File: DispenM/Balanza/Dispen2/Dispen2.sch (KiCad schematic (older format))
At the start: 13 parts, among them M1 Motor_Servo, U1 LoRa32U4, U2 DS3231MZ

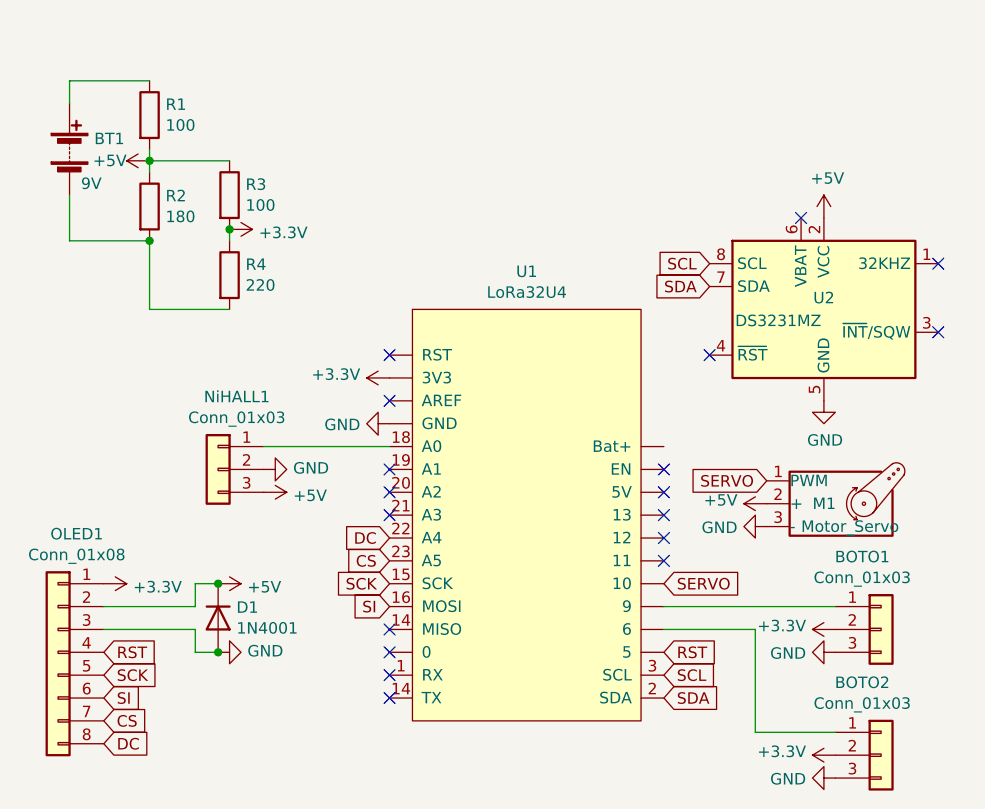
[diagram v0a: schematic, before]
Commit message: Actualizacion software y pcb
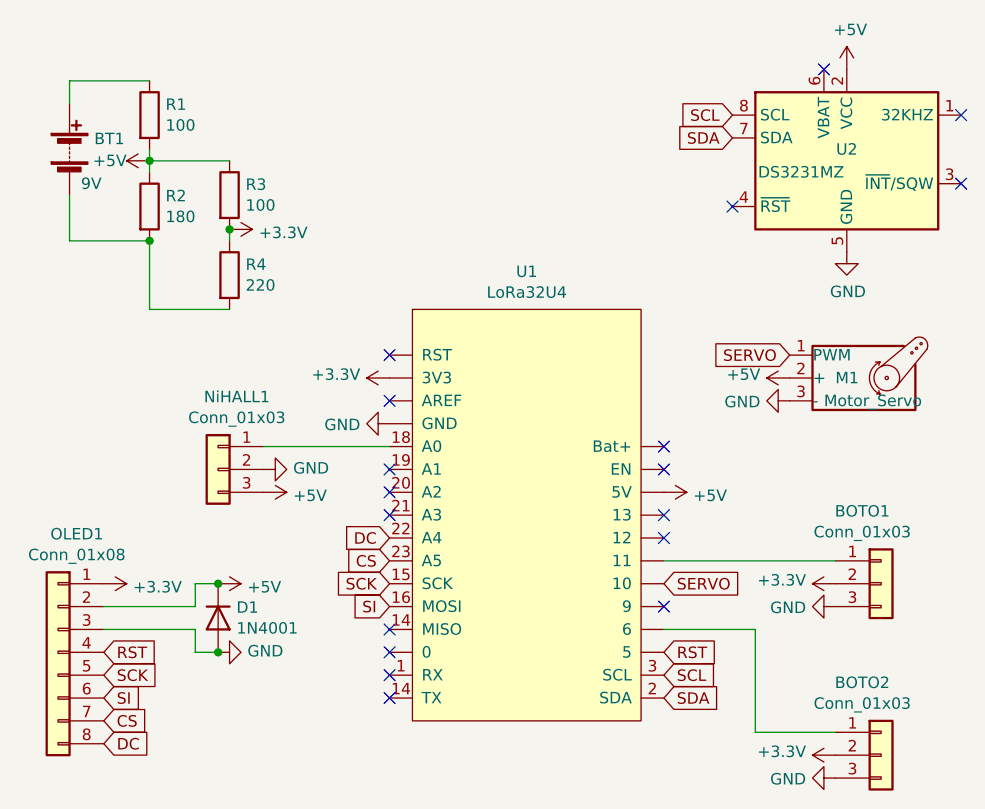
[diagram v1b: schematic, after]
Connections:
- net +5V: now also U1.~ (RST)
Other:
- moved on the sheet: BOTO1, M1, U2
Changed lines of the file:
@@
 $EndDescr
-$Comp
-L LoRa32U4:LoRa32U4 U1
-U 1 1 64849BFA
-P 5200 2750
-F 0 "U1" H 5200 3515 50  0000 C CNN
-F 1 "LoRa32U4" H 5200 3424 50  0000 C CNN
-F 2 "MODULOS:Lora32U4" H 5200 2750 50  0001 C CNN
-F 3 "" H 5200 2750 50  0001 C CNN
-	1    5200 2750
-	1    0    0    -1
-$EndComp
 $Comp
 L Motor:Motor_Servo M1
 U 1 1 6484B47B
-P 6550 3000
-F 0 "M1" H 6450 3000 50  0000 L CNN
-F 1 "Motor_Servo" H 6400 2900 50  0000 L CNN
-F 2 "Connector_PinHeader_2.54mm:PinHeader_1x03_P2.54mm_Vertical" H 6550 2810 50  0001 C CNN
-F 3 "http://forums.parallax.com/uploads/attachments/46831/74481.png" H 6550 2810 50  0001 C CNN
-	1    6550 3000
+P 6650 2450
+F 0 "M1" H 6550 2450 50  0000 L CNN
+F 1 "Motor_Servo" H 6500 2350 50  0000 L CNN
+F 2 "Connector_PinHeader_2.54mm:PinHeader_1x03_P2.54mm_Vertical" H 6650 2260 50  0001 C CNN
+F 3 "http://forums.parallax.com/uploads/attachments/46831/74481.png" H 6650 2260 50  0001 C CNN
+	1    6650 2450
 	1    0    0    -1
 $EndComp
@@
 L Timer_RTC:DS3231MZ U2
 U 1 1 6484C580
-P 6500 2150
-F 0 "U2" H 6500 2200 50  0000 C CNN
-F 1 "DS3231MZ" H 6300 2100 50  0000 C CNN
-F 2 "MODULOS:DS3231MH" H 6500 1650 50  0001 C CNN
-F 3 "http://datasheets.maximintegrated.com/en/ds/DS3231M.pdf" H 6500 1550 50  0001 C CNN
-	1    6500 2150
+P 6600 1500
+F 0 "U2" H 6600 1550 50  0000 C CNN
+F 1 "DS3231MZ" H 6400 1450 50  0000 C CNN
+F 2 "MODULOS:DS3231MH" H 6600 1000 50  0001 C CNN
+F 3 "http://datasheets.maximintegrated.com/en/ds/DS3231M.pdf" H 6600 900 50  0001 C CNN
+	1    6600 1500
 	1    0    0    -1
 $EndComp
@@
 L Connector_Generic:Conn_01x03 BOTO1
 U 1 1 6484ED92
-P 6750 3550
-F 0 "BOTO1" H 6668 3867 50  0000 C CNN
-F 1 "Conn_01x03" H 6668 3776 50  0000 C CNN
-F 2 "Connector_PinHeader_2.54mm:PinHeader_1x03_P2.54mm_Vertical" H 6750 3550 50  0001 C CNN
-F 3 "~" H 6750 3550 50  0001 C CNN
-	1    6750 3550
+P 6750 3350
+F 0 "BOTO1" H 6668 3667 50  0000 C CNN
+F 1 "Conn_01x03" H 6668 3576 50  0000 C CNN
+F 2 "Connector_PinHeader_2.54mm:PinHeader_1x03_P2.54mm_Vertical" H 6750 3350 50  0001 C CNN
+F 3 "~" H 6750 3350 50  0001 C CNN
+	1    6750 3350
 	1    0    0    -1
 $EndComp
@@
 L power:+3.3V #PWR0102
 U 1 1 648545ED
-P 6550 3550
-F 0 "#PWR0102" H 6550 3400 50  0001 C CNN
-F 1 "+3.3V" V 6565 3678 50  0000 L CNN
-F 2 "" H 6550 3550 50  0001 C CNN
-F 3 "" H 6550 3550 50  0001 C CNN
-	1    6550 3550
+P 6550 3350
+F 0 "#PWR0102" H 6550 3200 50  0001 C CNN
+F 1 "+3.3V" V 6565 3478 50  0000 L CNN
+F 2 "" H 6550 3350 50  0001 C CNN
+F 3 "" H 6550 3350 50  0001 C CNN
+	1    6550 3350
 	0    -1   -1   0
 $EndComp
@@
 L power:+5V #PWR0104
 U 1 1 64856200
-P 6250 3000
-F 0 "#PWR0104" H 6250 2850 50  0001 C CNN
-F 1 "+5V" V 6265 3128 50  0000 L CNN
-F 2 "" H 6250 3000 50  0001 C CNN
-F 3 "" H 6250 3000 50  0001 C CNN
-	1    6250 3000
+P 6350 2450
+F 0 "#PWR0104" H 6350 2300 50  0001 C CNN
+F 1 "+5V" V 6365 2578 50  0000 L CNN
+F 2 "" H 6350 2450 50  0001 C CNN
+F 3 "" H 6350 2450 50  0001 C CNN
+	1    6350 2450
 	0    -1   -1   0
 $EndComp
@@
 L power:+5V #PWR0105
 U 1 1 64856E0D
-P 6500 1750
-F 0 "#PWR0105" H 6500 1600 50  0001 C CNN
-F 1 "+5V" H 6515 1923 50  0000 C CNN
-F 2 "" H 6500 1750 50  0001 C CNN
-F 3 "" H 6500 1750 50  0001 C CNN
-	1    6500 1750
+P 6600 1100
+F 0 "#PWR0105" H 6600 950 50  0001 C CNN
+F 1 "+5V" H 6615 1273 50  0000 C CNN
+F 2 "" H 6600 1100 50  0001 C CNN
+F 3 "" H 6600 1100 50  0001 C CNN
+	1    6600 1100
 	1    0    0    -1
 $EndComp
@@
 	0    1    1    0
 $EndComp
-NoConn ~ 7000 1950
-NoConn ~ 7000 2250
-NoConn ~ 6000 2350
+NoConn ~ 7100 1300
+NoConn ~ 7100 1600
+NoConn ~ 6100 1700
 $Comp
 L power:GND #PWR0107
@@
 L power:GND #PWR0109
 U 1 1 6485B66E
-P 6500 2550
-F 0 "#PWR0109" H 6500 2300 50  0001 C CNN
-F 1 "GND" H 6505 2377 50  0000 C CNN
-F 2 "" H 6500 2550 50  0001 C CNN
-F 3 "" H 6500 2550 50  0001 C CNN
-	1    6500 2550
+P 6600 1900
+F 0 "#PWR0109" H 6600 1650 50  0001 C CNN
+F 1 "GND" H 6605 1727 50  0000 C CNN
+F 2 "" H 6600 1900 50  0001 C CNN
+F 3 "" H 6600 1900 50  0001 C CNN
+	1    6600 1900
 	1    0    0    -1
 $EndComp
@@
 L power:GND #PWR0110
 U 1 1 6485BFB9
-P 6550 3650
-F 0 "#PWR0110" H 6550 3400 50  0001 C CNN
-F 1 "GND" V 6555 3522 50  0000 R CNN
-F 2 "" H 6550 3650 50  0001 C CNN
-F 3 "" H 6550 3650 50  0001 C CNN
-	1    6550 3650
+P 6550 3450
+F 0 "#PWR0110" H 6550 3200 50  0001 C CNN
+F 1 "GND" V 6555 3322 50  0000 R CNN
+F 2 "" H 6550 3450 50  0001 C CNN
+F 3 "" H 6550 3450 50  0001 C CNN
+	1    6550 3450
 	0    1    1    0
 $EndComp
@@
 L power:GND #PWR0112
 U 1 1 6485CF38
-P 6250 3100
-F 0 "#PWR0112" H 6250 2850 50  0001 C CNN
-F 1 "GND" V 6255 2972 50  0000 R CNN
-F 2 "" H 6250 3100 50  0001 C CNN
-F 3 "" H 6250 3100 50  0001 C CNN
-	1    6250 3100
+P 6350 2550
+F 0 "#PWR0112" H 6350 2300 50  0001 C CNN
+F 1 "GND" V 6355 2422 50  0000 R CNN
+F 2 "" H 6350 2550 50  0001 C CNN
+F 3 "" H 6350 2550 50  0001 C CNN
+	1    6350 2550
 	0    1    1    0
 $EndComp
@@
 Text GLabel 5800 3350 2    50   Input ~ 0
 SERVO
-Text GLabel 6000 1950 0    50   Input ~ 0
+Text GLabel 6100 1300 0    50   Input ~ 0
 SCL
-Text GLabel 6000 2050 0    50   Input ~ 0
+Text GLabel 6100 1400 0    50   Input ~ 0
 SDA
-Text GLabel 6250 2900 0    50   Input ~ 0
+Text GLabel 6350 2350 0    50   Input ~ 0
 SERVO
 $Comp
@@
 Wire Wire Line
 	6200 4000 6550 4000
-NoConn ~ 5800 3250
+NoConn ~ 5800 3450
 NoConn ~ 5800 3150
 NoConn ~ 5800 3050
-NoConn ~ 5800 2950
 NoConn ~ 5800 2850
+NoConn ~ 5800 2750
 NoConn ~ 4600 2350
 NoConn ~ 4600 2550
@@
 NoConn ~ 4600 3750
 NoConn ~ 4600 3850
-NoConn ~ 6400 1750
+NoConn ~ 6500 1100
 $Comp
 L Device:Battery BT1
@@
 	0    -1   -1   0
 $EndComp
-Wire Wire Line
-	5800 3450 6550 3450
 NoConn ~ 4600 2850
 NoConn ~ 4600 2950
 NoConn ~ 4600 3050
+Wire Wire Line
+	6550 3250 5800 3250
+$Comp
+L LoRa32U4:LoRa32U4 U1
+U 1 1 64BFF81C
+P 5200 2750
+F 0 "U1" H 5200 3515 50  0000 C CNN
+F 1 "LoRa32U4" H 5200 3424 50  0000 C CNN
+F 2 "MODULOS:Lora32U4" H 5200 2750 50  0001 C CNN
+F 3 "" H 5200 2750 50  0001 C CNN
+	1    5200 2750
+	1    0    0    -1
+$EndComp
+$Comp
+L power:+5V #PWR0118
+U 1 1 64C03C45
+P 5800 2950
+F 0 "#PWR0118" H 5800 2800 50  0001 C CNN
+F 1 "+5V" V 5815 3078 50  0000 L CNN
+F 2 "" H 5800 2950 50  0001 C CNN
+F 3 "" H 5800 2950 50  0001 C CNN
+	1    5800 2950
+	0    1    1    0
+$EndComp
 $EndSCHEMATC
